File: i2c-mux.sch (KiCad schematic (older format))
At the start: 20 parts, among them J501 SMBUS, J502 SMBUS, J503 SMBUS, J504 SMBUS, U501 LTC4306CGN

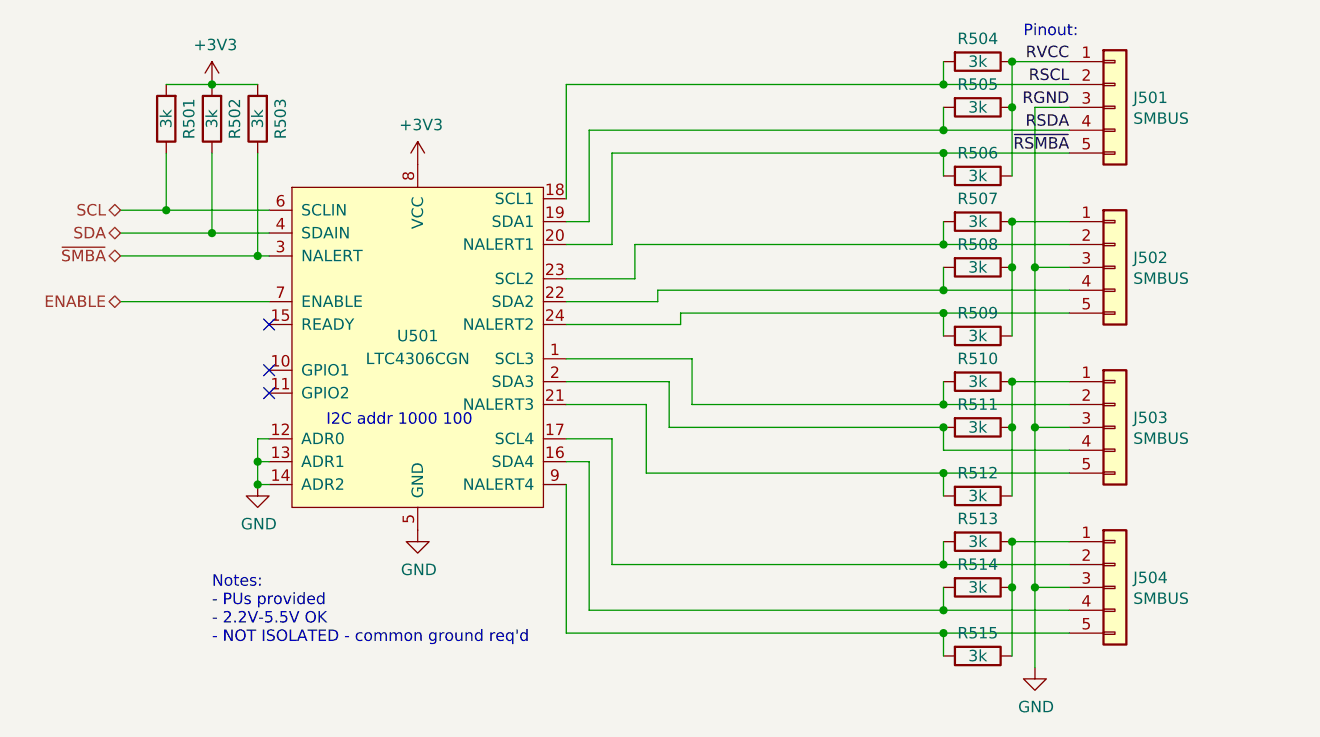
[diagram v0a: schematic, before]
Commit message: SMD resistor packs @ fan controller, i2c mux
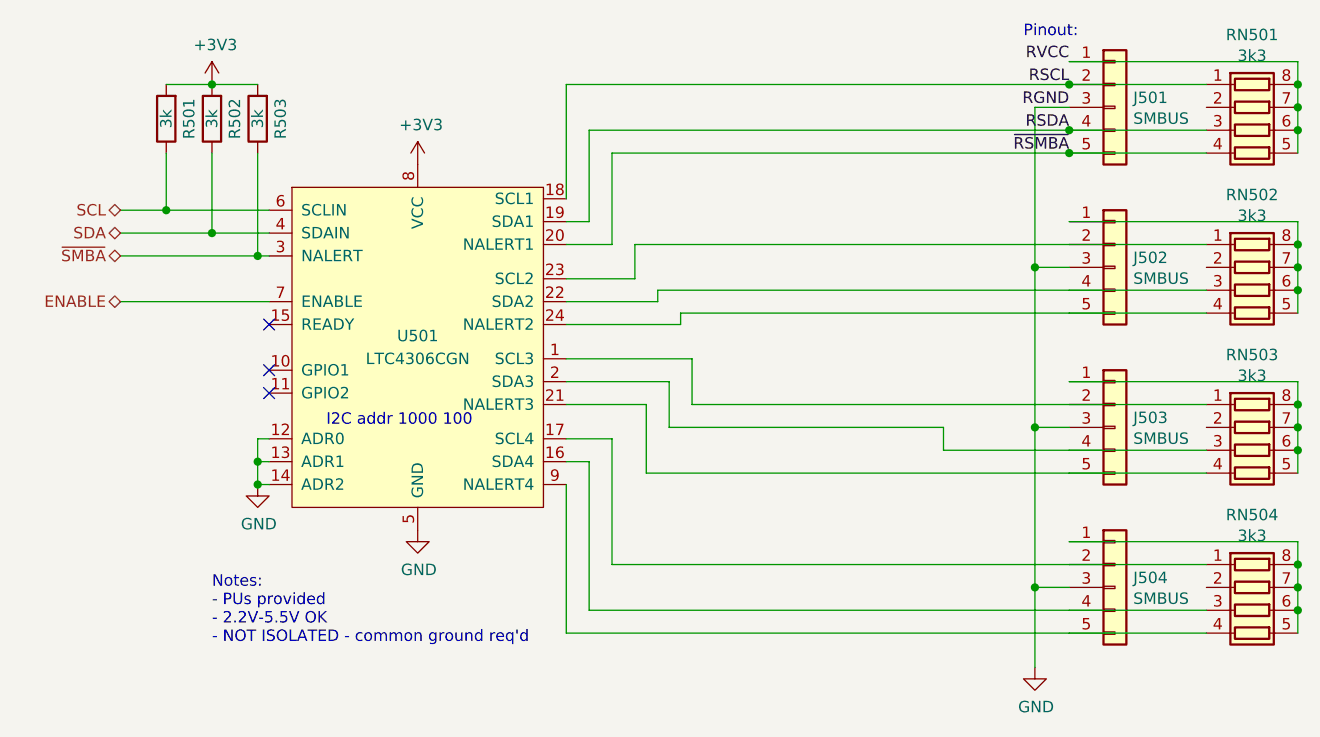
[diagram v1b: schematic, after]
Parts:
- removed R504, R505, R506, R507, R508, R509, R510, R511, R512, R513, R514, R515: 3k, Resistor_SMD:R_0603_1608Metric, symbol Device:R
- added RN501, RN502, RN503, RN504: 3k3, Resistor_SMD:R_Array_Convex_4x1206, symbol Device:R_Pack04
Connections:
- net RSCL: now also RN501.1 (R1.1)
- net RSDA: now also RN501.3 (R3.1)
- net RVCC: now also RN501.5 (R4.2), RN501.6 (R3.2), RN501.7 (R2.2), RN501.8 (R1.2)
- net ~RSMBA: now also RN501.4 (R4.1)
- net at J502.1 (Pin_1): now also RN502.5 (R4.2), RN502.6 (R3.2), RN502.7 (R2.2), RN502.8 (R1.2)
- net at J502.2 (Pin_2), U501.23 (SCL2): now also RN502.1 (R1.1)
- net at J502.4 (Pin_4), U501.22 (SDA2): now also RN502.3 (R3.1)
- net at J502.5 (Pin_5), U501.24 (NALERT2): now also RN502.4 (R4.1)
- net at J503.1 (Pin_1): now also RN503.5 (R4.2), RN503.6 (R3.2), RN503.7 (R2.2), RN503.8 (R1.2)
- net at J503.2 (Pin_2), U501.1 (SCL3): now also RN503.1 (R1.1)
- net at J503.4 (Pin_4), U501.2 (SDA3): now also RN503.3 (R3.1)
- net at J503.5 (Pin_5), U501.21 (NALERT3): now also RN503.4 (R4.1)
- net at J504.1 (Pin_1): now also RN504.5 (R4.2), RN504.6 (R3.2), RN504.7 (R2.2), RN504.8 (R1.2)
- net at J504.2 (Pin_2), U501.17 (SCL4): now also RN504.1 (R1.1)
- net at J504.4 (Pin_4), U501.16 (SDA4): now also RN504.3 (R3.1)
- net at J504.5 (Pin_5), U501.9 (NALERT4): now also RN504.4 (R4.1)
